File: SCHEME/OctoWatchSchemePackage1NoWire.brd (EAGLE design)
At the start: 35 x 34 mm, 24 parts, among them IC1 TP4056, IC2 DS1302, J1 0475900001, Y2 32.768kHz

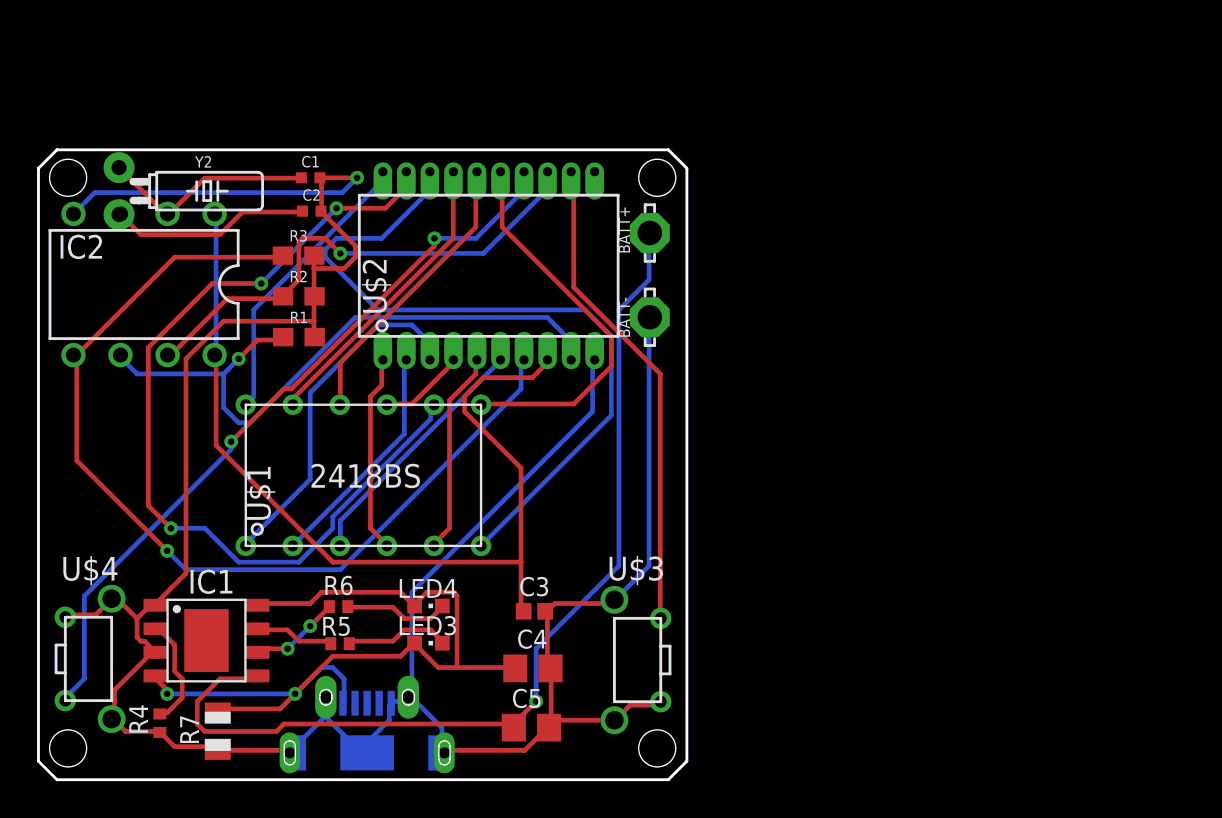
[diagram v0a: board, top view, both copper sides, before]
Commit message: Finalizing...
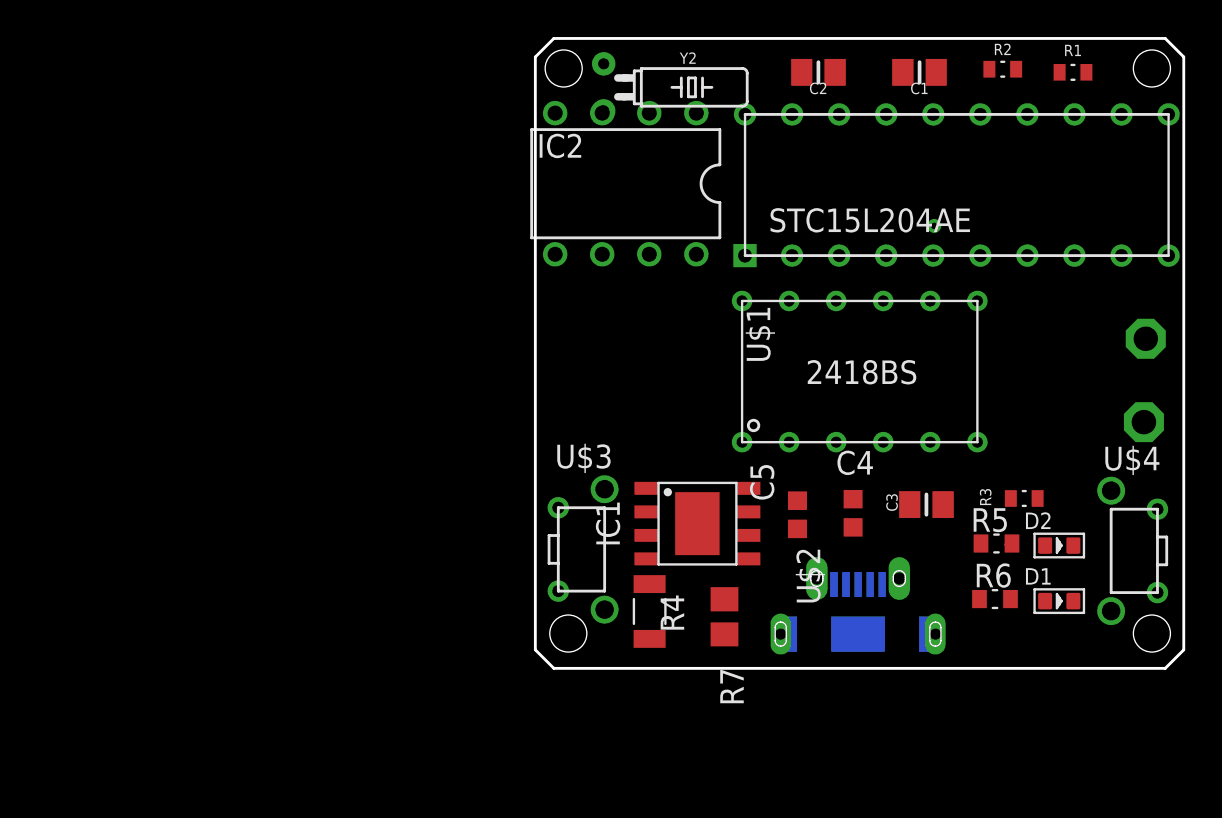
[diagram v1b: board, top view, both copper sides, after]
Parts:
- removed LED3, LED4: (no value), adafruit:CHIPLED_0603
- added D1: SMD-LED-CLEAR-BLUE(0603), SMD-LED-CLEAR-BLUE_0603_:LED-0603
- added D2: LED-SMD-RED-DIFFUSED(0603), LED-SMD-RED-DIFFUSED_0603_:LED-0603
- C1, C2: value 22pF -> CL21C220JBANNNC; device SparkFun-Capacitors:0402-TIGHT -> CL21C220JBANNNC:CAPC2012X140N
- C3: value 0.1uF -> CL21B104KCFNNNE; device SparkFun-Capacitors:0402 -> CL21B104KCFNNNE:CAPC2012X140N
- C4, C5: device rcl:C0805 -> GRT188R61E106ME13D:CAPC1608X100N
- R1, R2, R3: value 10k -> ERA3AEB103V; device SparkFun-Resistors:0603 -> ERA3AEB103V:RES_ERA3AEB103V
- R4: device rcl:R0402 -> AC1206FR-073K9L:RESC3116X65N
- R5, R6: device rcl:R0402 -> ERJ-PB3B1001V:RESC1608X55N
- R7: device adafruit:R0805 -> rcl:R0805
- U$2: device OctoWatch:STC15F204AE -> OctoWatch:STC15F204AE2
- moved U$4 77.0 mm to (71.8, 27.2), turned to 0 degrees
- moved R1 44.2 mm to (58.2, 55.3), turned to 180 degrees
- moved R3 41.3 mm to (55.6, 32.3), turned to 180 degrees
- moved R2 39.9 mm to (54.5, 55.5)
- moved R5 35.8 mm to (54.1, 29.9)
- moved R6 35.4 mm to (54.0, 26.9)
- moved C1 33.4 mm to (50.0, 55.3), turned to 180 degrees
- moved U$2 32.3 mm to (50.7, 58.1)
- moved BATT+ 28.6 mm to (62.1, 36.4), flipped to the bottom, turned to 0 degrees
- moved C2 28.4 mm to (44.5, 55.3), turned to 180 degrees
- moved R7 28.0 mm to (39.4, 25.9), turned to 270 degrees
- moved U$1 27.4 mm to (48.0, 48.0)
- moved J1 27.3 mm to (46.6, 25.0)
- moved IC1 27.2 mm to (38.0, 30.9)
- moved R4 27.1 mm to (35.4, 26.2)
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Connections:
- removed net N$32: C4.1, IC1.4, IC1.8, J1.1, LED3.A, LED4.A, R7.2
- new net N$11: IC2.-RST, R3.2, U$2.P$7
- new net SHIELD: J1.SH1, J1.SH2, J1.SH3, J1.SH4, J1.SH5
- net BATT+: now also R1.2, R2.2, R3.1, R7.2
- net GND: now also J1.1; no longer J1.5, J1.SH1, J1.SH2, J1.SH3, J1.SH4, J1.SH5, R1.2, R2.2, R3.2, R7.1
- net N$14: now also C4.1, D1.-, D2.-, IC1.4, IC1.8, J1.5, R7.1; no longer IC2.-RST, R3.1, U$2.P$7
- net N$27: now also D1.+; no longer LED4.C
- net N$29: now also D2.+; no longer LED3.C
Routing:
- net GND: track 153.8 -> 1.41 mm, vias 1 -> 0
- net N$18: track 52.2 -> 0.22 mm, vias 1 -> 0
- net N$14: track 51.4 -> 0.23 mm, vias 1 -> 0
- net BATT+: track 50.0 -> 0.00 mm
- net N$21: track 47.8 -> 0.00 mm, vias 3 -> 0
- net N$32: track 46.9 -> 0.00 mm, vias 2 -> 0
- net N$19: track 40.4 -> 0.00 mm, vias 2 -> 0
- net N$6: track 39.8 -> 0.00 mm
- net N$17: track 34.9 -> 0.00 mm, vias 1 -> 0
- net N$10: track 27.0 -> 0.00 mm, vias 1 -> 0
- net N$20: track 26.1 -> 0.14 mm
- net N$12: track 20.9 -> 0.00 mm
- net N$1: track 19.0 -> 0.00 mm
- net N$8: track 16.2 -> 0.00 mm
- net N$7: track 15.6 -> 0.00 mm
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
